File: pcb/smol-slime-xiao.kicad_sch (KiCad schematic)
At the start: 11 parts, among them J1 Conn_01x02, U1 ICM-45686, U3 1532H, U4 XIAO-nRF52840-SMD

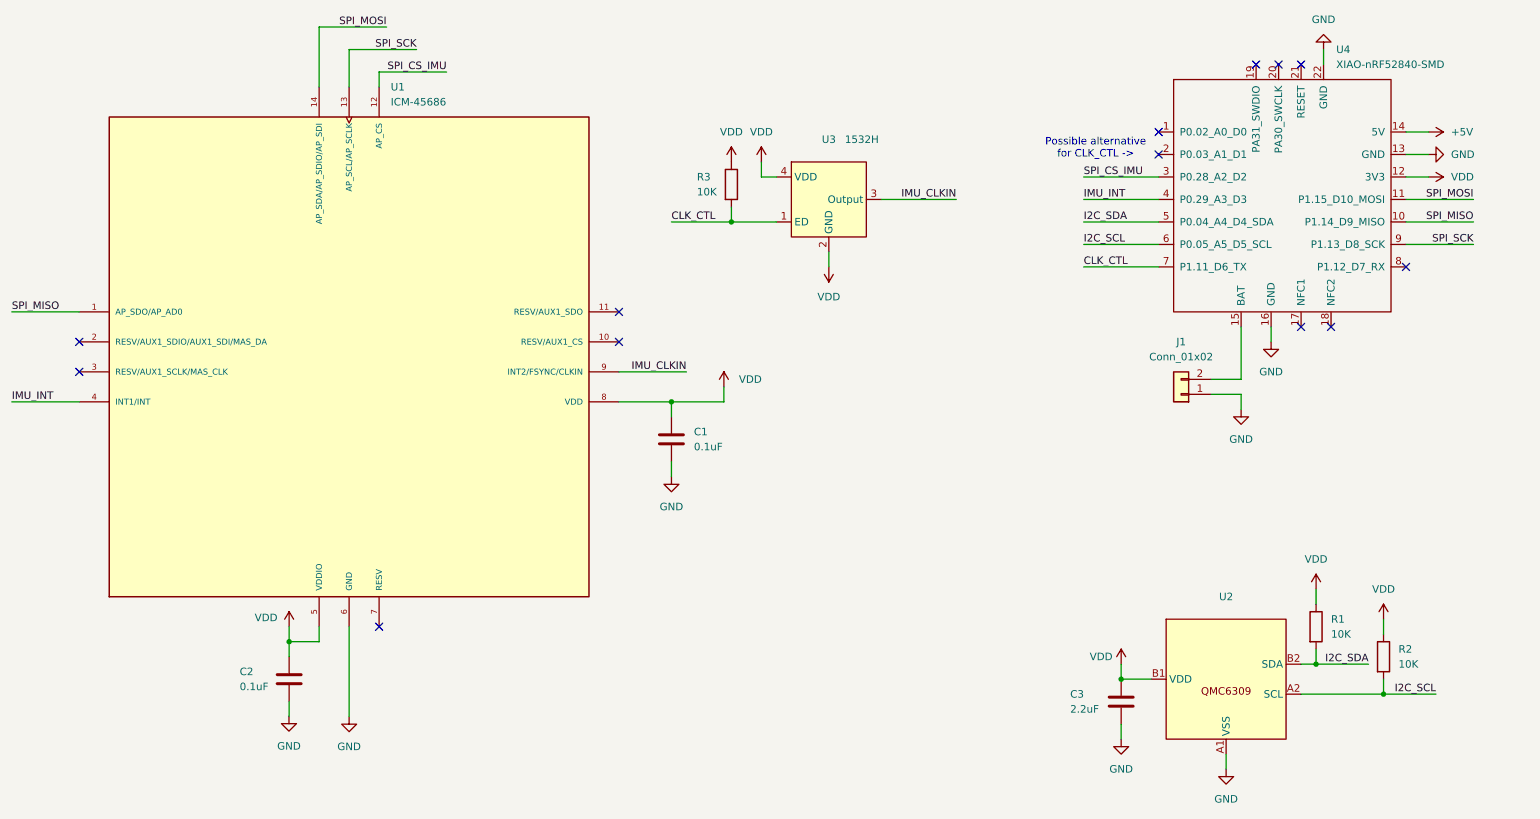
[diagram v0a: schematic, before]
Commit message: Add MCU connectors
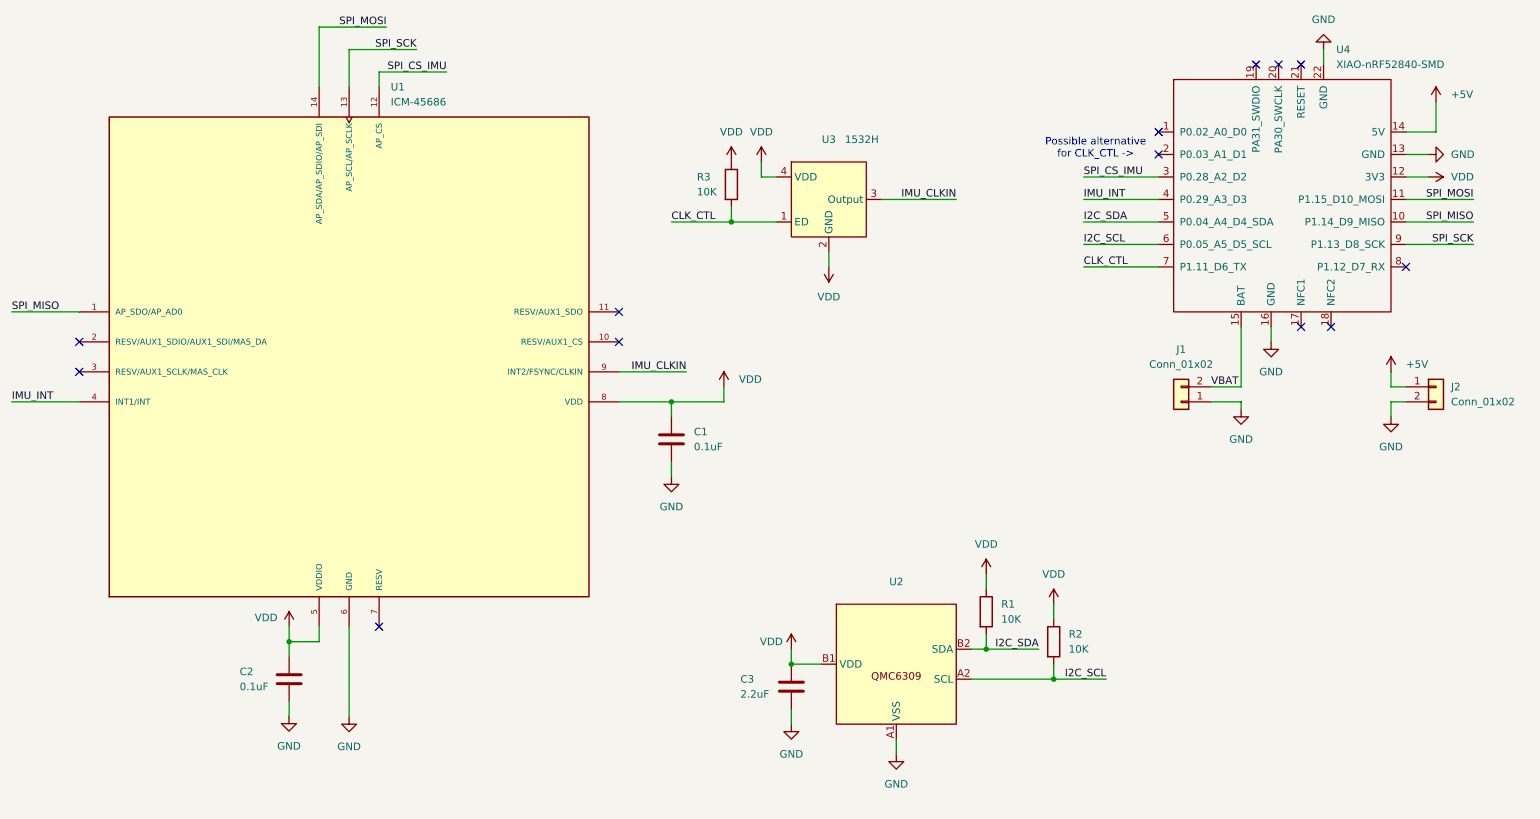
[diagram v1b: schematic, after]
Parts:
- added J2: Conn_01x02, symbol Connector_Generic:Conn_01x02
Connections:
- net +5V: now also J2.1 (Pin_1)
- net GND: now also J2.2 (Pin_2)
- net VBAT: now reaches J1.2 (Pin_2), U4.15 (BAT)
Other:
- moved on the sheet: C3, J1, R1, R2, U2
